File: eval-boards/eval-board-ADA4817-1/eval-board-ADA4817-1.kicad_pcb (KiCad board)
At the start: 2 copper layers, 36 parts, among them U1 ADA4817-1

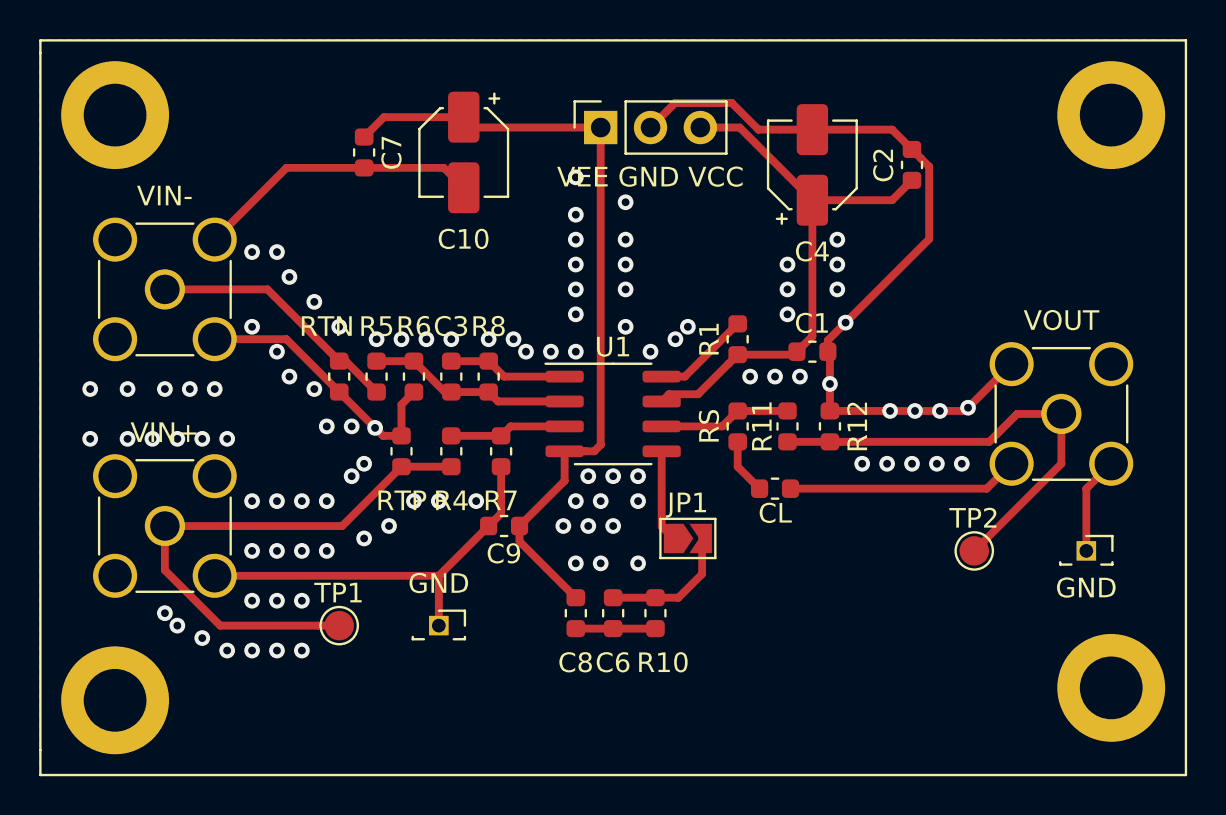
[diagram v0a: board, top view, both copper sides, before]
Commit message: update-version
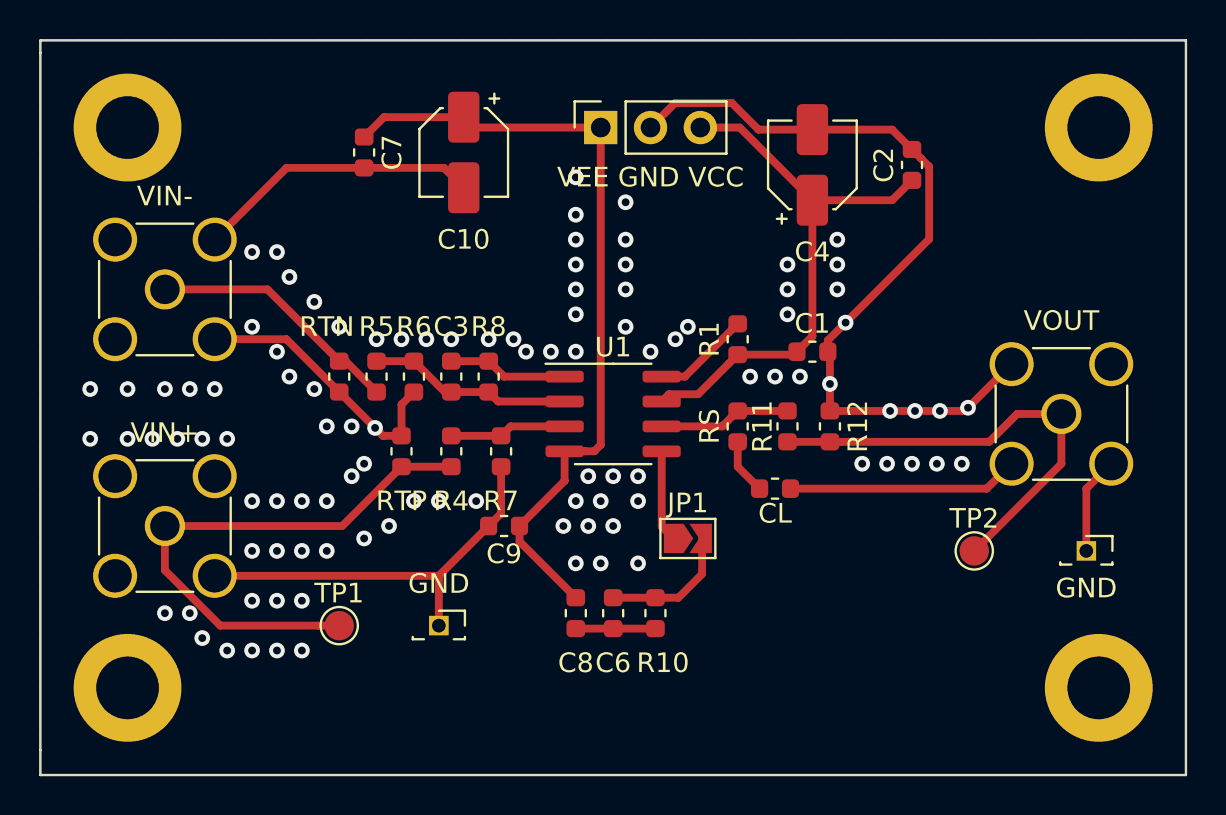
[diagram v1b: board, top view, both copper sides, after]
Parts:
- moved REF** 0.90 mm to (107.3, 132.1)
- moved REF** 0.90 mm to (156.8, 103.5)
- moved REF** 0.90 mm to (107.3, 103.5)
- moved REF** 0.63 mm to (156.8, 132.1)
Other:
- board outline added: 58.4 x 37.5 mm
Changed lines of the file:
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@@
   (general
     (thickness 1.6)
-    (drawings 6)
+    (drawings 10)
     (tracks 215)
     (zones 0)
@@
   )
   (setup
-    (last_trace_width 0.4)
+    (last_trace_width 0.25)
     (user_trace_width 0.4)
     (trace_clearance 0.2)
@@
     (solder_mask_min_width 0.25)
     (aux_axis_origin 0 0)
-    (visible_elements FFFFFF7F)
+    (visible_elements 7FFFFFFF)
     (pcbplotparams
-      (layerselection 0x010fc_ffffffff)
+      (layerselection 0x010f0_ffffffff)
       (usegerberextensions false)
       (usegerberattributes false)
@@
   )
   (module MountingHole:MountingHole_3.2mm_M3_ISO14580_Pad (layer F.Cu)
-    (at 106.68 132.715)
+    (at 107.315 132.08)
     (descr "Mounting Hole 3.2mm, M3, ISO14580")
     (tags "mounting hole 3.2mm m3 iso14580")
@@
   )
   (module MountingHole:MountingHole_3.2mm_M3_ISO14580_Pad (layer F.Cu)
-    (at 157.48 132.08)
+    (at 156.845 132.08)
     (descr "Mounting Hole 3.2mm, M3, ISO14580")
     (tags "mounting hole 3.2mm m3 iso14580")
@@
   )
   (module MountingHole:MountingHole_3.2mm_M3_ISO14580_Pad (layer F.Cu)
-    (at 157.48 102.87)
+    (at 156.845 103.505)
     (descr "Mounting Hole 3.2mm, M3, ISO14580")
     (tags "mounting hole 3.2mm m3 iso14580")
@@
   )
   (module MountingHole:MountingHole_3.2mm_M3_ISO14580_Pad (layer F.Cu)
-    (at 106.68 102.87)
+    (at 107.315 103.505)
     (descr "Mounting Hole 3.2mm, M3, ISO14580")
     (tags "mounting hole 3.2mm m3 iso14580")
@@
     )
   )
+  (gr_line (start 102.87 135.255) (end 102.87 136.525) (layer F.SilkS) (width 0.12))
+  (gr_line (start 102.87 99.06) (end 102.87 99.695) (layer F.SilkS) (width 0.12))
+  (gr_line (start 102.87 99.695) (end 102.87 135.255) (layer F.SilkS) (width 0.12))
+  (gr_line (start 102.87 99.06) (end 102.87 136.525) (layer Edge.Cuts) (width 0.05))
+  (gr_line (start 161.29 99.06) (end 102.87 99.06) (layer Edge.Cuts) (width 0.05))
+  (gr_line (start 161.29 136.525) (end 161.29 99.06) (layer Edge.Cuts) (width 0.05))
+  (gr_line (start 102.87 136.525) (end 161.29 136.525) (layer Edge.Cuts) (width 0.05))
   (gr_line (start 161.29 136.525) (end 102.87 136.525) (layer F.SilkS) (width 0.12))
   (gr_line (start 161.29 99.06) (end 161.29 136.525) (layer F.SilkS) (width 0.12))
-  (gr_line (start 102.87 135.255) (end 102.87 136.525) (layer F.SilkS) (width 0.12))
-  (gr_line (start 102.87 99.06) (end 102.87 99.695) (layer F.SilkS) (width 0.12))
   (gr_line (start 161.29 99.06) (end 102.87 99.06) (layer F.SilkS) (width 0.12))
-  (gr_line (start 102.87 99.695) (end 102.87 135.255) (layer F.SilkS) (width 0.12))
   (segment (start 137.968388 115.549112) (end 138.43 115.0875) (width 0.4) (layer F.Cu) (net 1))
   (segment (start 136.41321 117.10429) (end 137.968388 115.549112) (width 0.4) (layer F.Cu) (net 1))
@@
   (via (at 127 114.3) (size 0.8) (drill 0.4) (layers F.Cu B.Cu) (net 2))
   (via (at 109.22 128.27) (size 0.8) (drill 0.4) (layers F.Cu B.Cu) (net 2))
-  (via (at 109.855 128.905) (size 0.8) (drill 0.4) (layers F.Cu B.Cu) (net 2))
+  (via (at 110.49 128.27) (size 0.8) (drill 0.4) (layers F.Cu B.Cu) (net 2))
   (via (at 111.125 129.54) (size 0.8) (drill 0.4) (layers F.Cu B.Cu) (net 2))
   (via (at 112.395 130.175) (size 0.8) (drill 0.4) (layers F.Cu B.Cu) (net 2))
